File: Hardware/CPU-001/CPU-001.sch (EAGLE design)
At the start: 93 parts, among them IC1 IS42S16800F-7TL, IC2 NCV1117ST33T3G, IC3 TLV71318PQDBVRQ1, J1 10144517-042802LF, J2 10144518-041802LF, J3 10144517-042802LF, J4 10144518-041802LF, J6 2X5_0.05_SWD, U1 ATSAMV71Q19B-AABT, U2 ATA6561-GAQW-N, U3 ICP-10111, U4 PCA9306, U7 ATA6561-GAQW-N

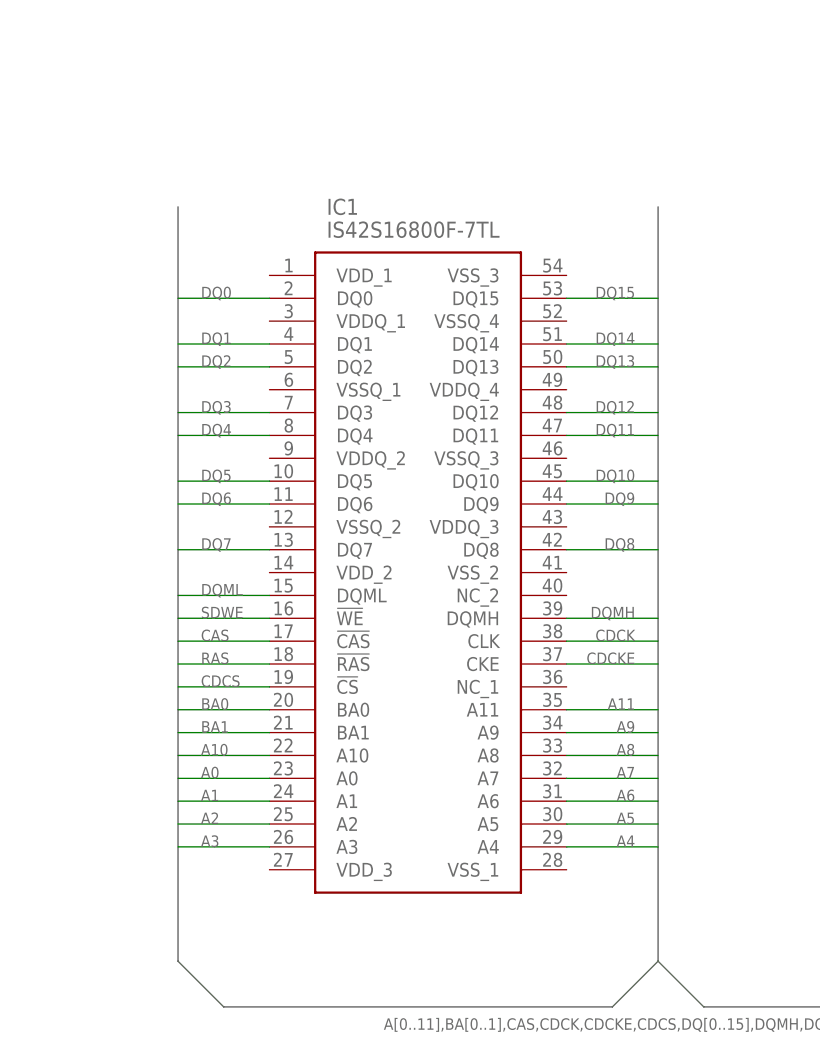
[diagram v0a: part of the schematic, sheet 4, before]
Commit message: updates to CPU-001 and DBG-001
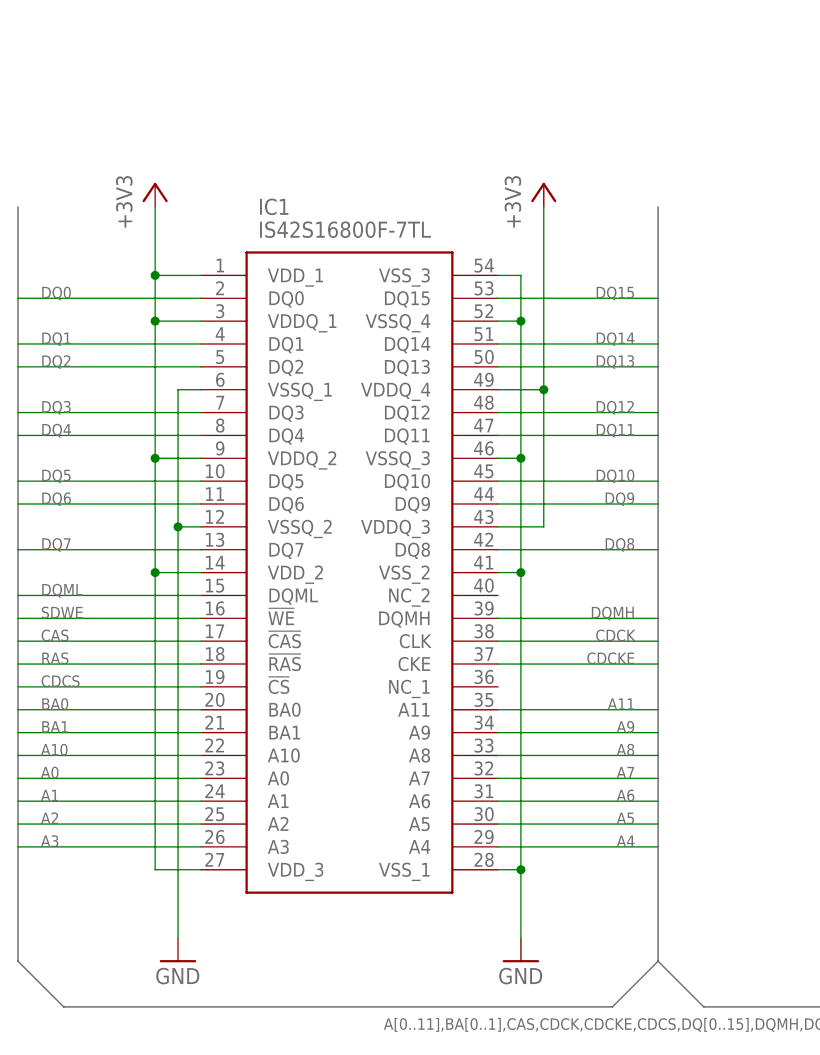
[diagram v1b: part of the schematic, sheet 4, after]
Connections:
- net +3V3: now also IC1.VDDQ_1, IC1.VDDQ_2, IC1.VDDQ_3, IC1.VDDQ_4, IC1.VDD_1, IC1.VDD_2, IC1.VDD_3
- net GND: now also IC1.VSSQ_1, IC1.VSSQ_2, IC1.VSSQ_3, IC1.VSSQ_4, IC1.VSS_1, IC1.VSS_2, IC1.VSS_3
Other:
- moved on the sheet: IC1
